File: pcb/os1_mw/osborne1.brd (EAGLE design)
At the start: 148 x 100 mm, 19 parts

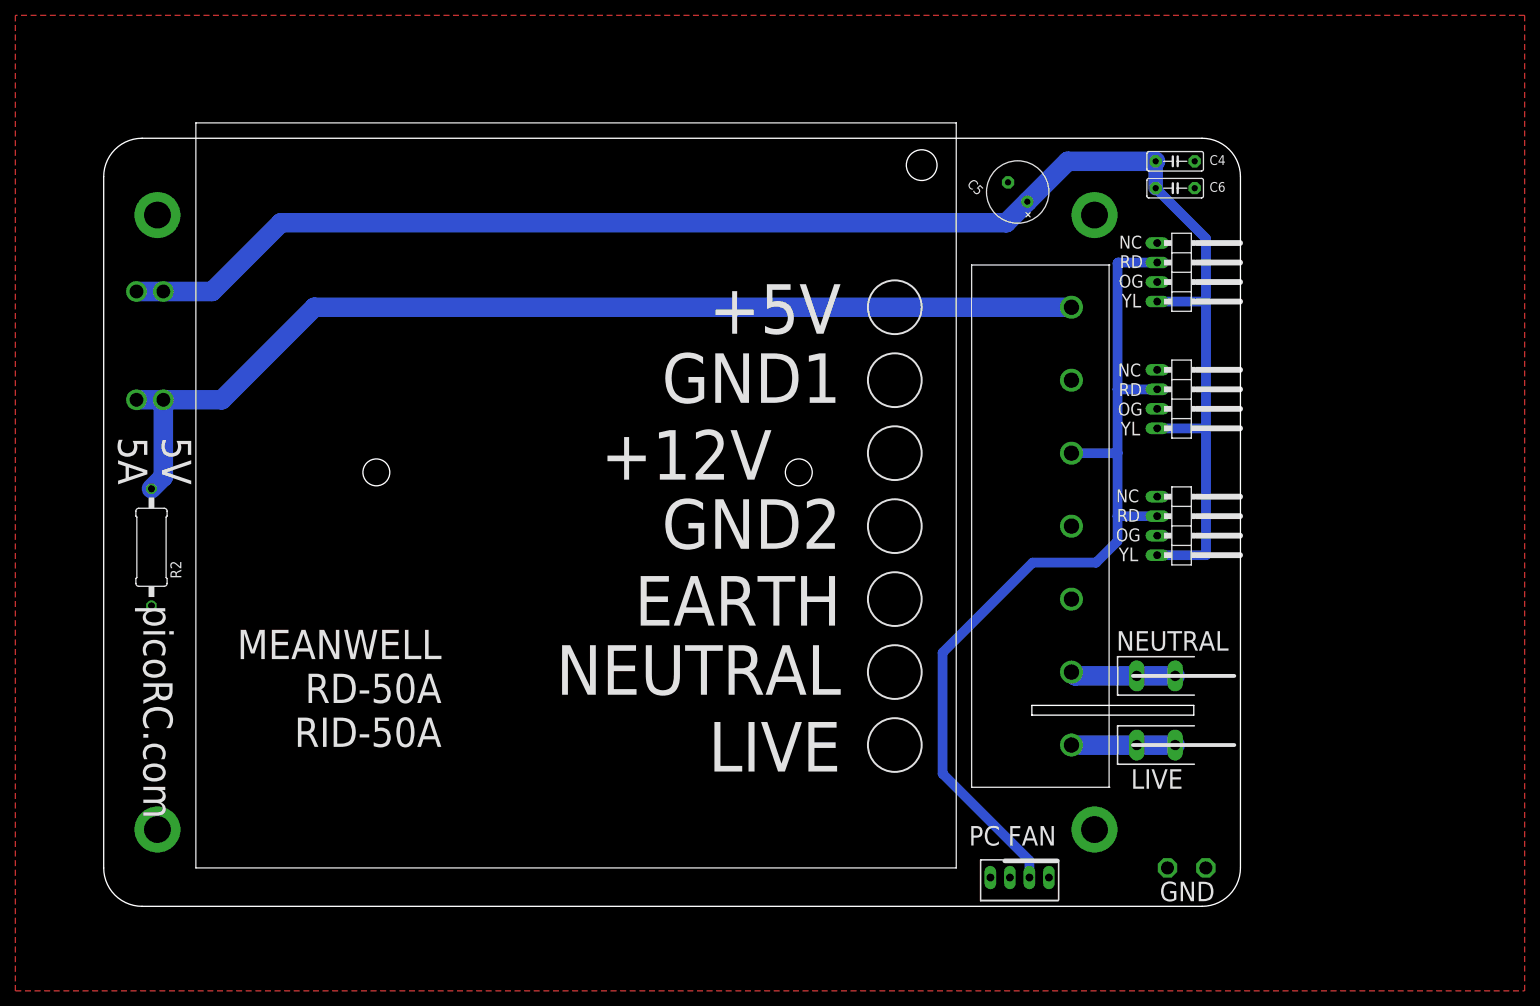
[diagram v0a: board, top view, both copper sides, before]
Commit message: mw os1
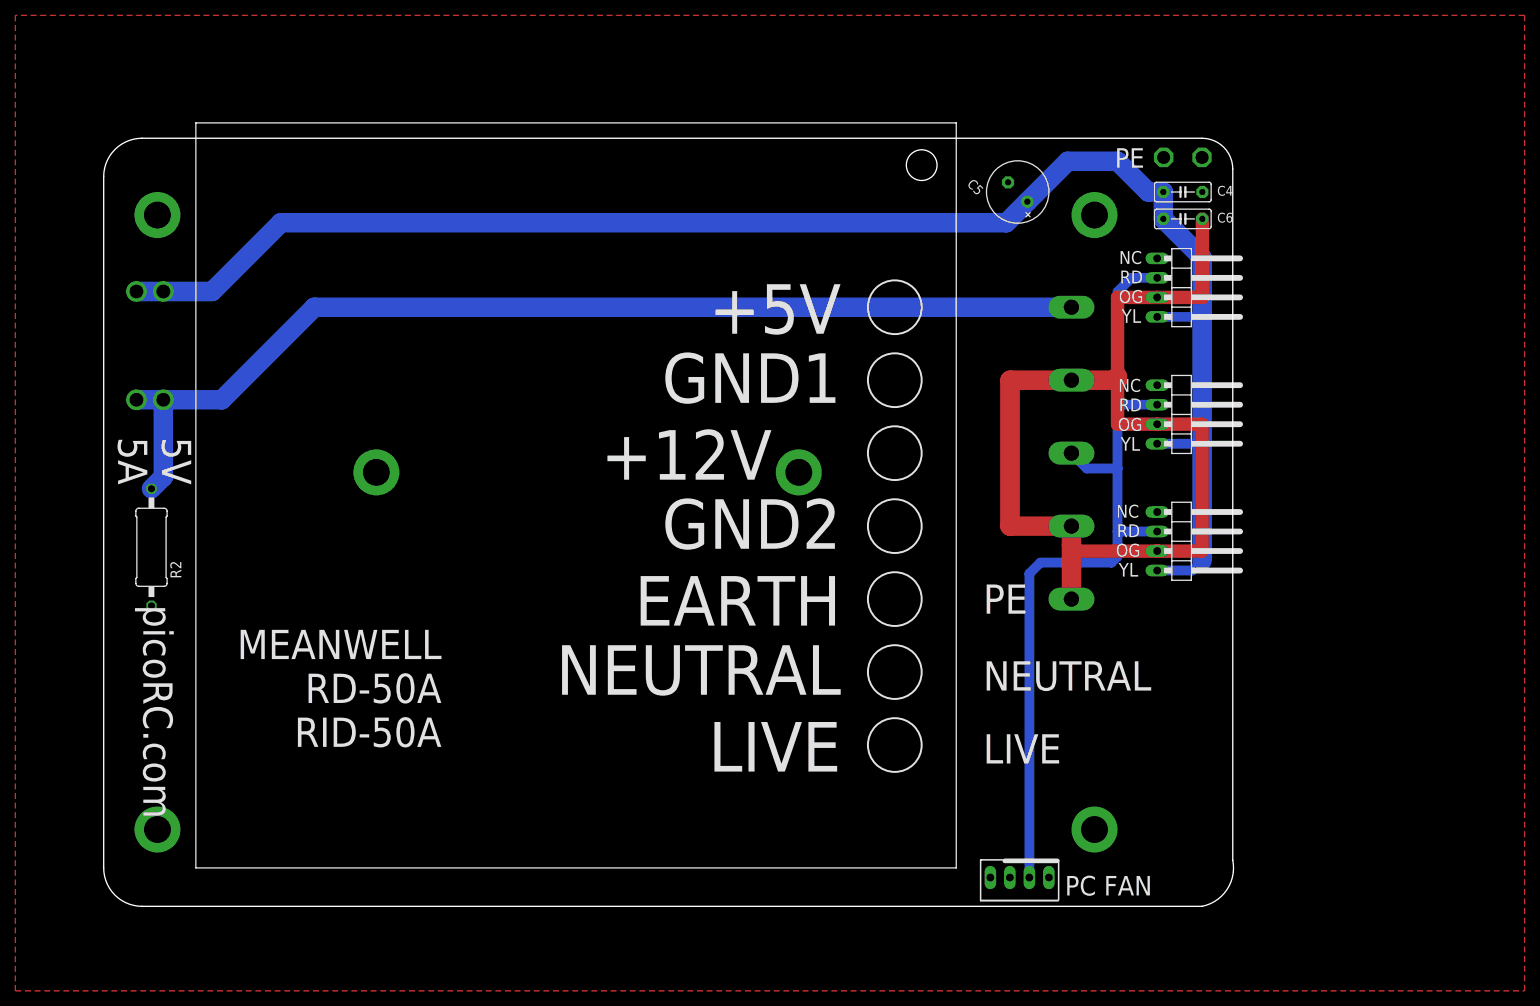
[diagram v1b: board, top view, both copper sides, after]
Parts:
- removed U$14, U$3: 28FLAG, blade:2.8FLAG
- U$1: device apricot:MEANWELL_RD50 -> os1:MEANWELL_RD50
- U$2: value TERM9.5 -> TERM_RD50; device os1:TERMINAL9500 -> os1:TERMINAL9500_NOMAINS
- moved TP1 92.5 mm to (138.0, 97.5)
- moved TP2 92.5 mm to (143.0, 97.5)
- moved C4 4.12 mm to (140.5, 93.0)
- moved C6 4.12 mm to (140.5, 89.5)
- moved JP1 2.00 mm to (141.0, 80.5)
- moved JP2 2.00 mm to (141.0, 47.5)
- moved JP3 2.00 mm to (141.0, 64.0)
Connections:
- removed net LIVE: U$2.P$7, U$3.P$1, U$3.P$2
- removed net NEUTRAL: U$14.P$1, U$14.P$2, U$2.P$6
- net GND: now also U$1.P$1, U$1.P$2
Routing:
- net GND: track 0.00 -> 134.0 mm
- net NEUTRAL: track 13.7 -> 0.00 mm
- net LIVE: track 13.5 -> 0.00 mm
- net +12V: track 120.5 -> 109.5 mm
- net +5V: track 212.8 -> 211.0 mm
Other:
- board size 148 x 100 mm -> 147.1 x 100 mm
- board text added: "PE"
